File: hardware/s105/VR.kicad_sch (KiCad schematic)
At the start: 18 parts, among them Q19 ., U3 case only

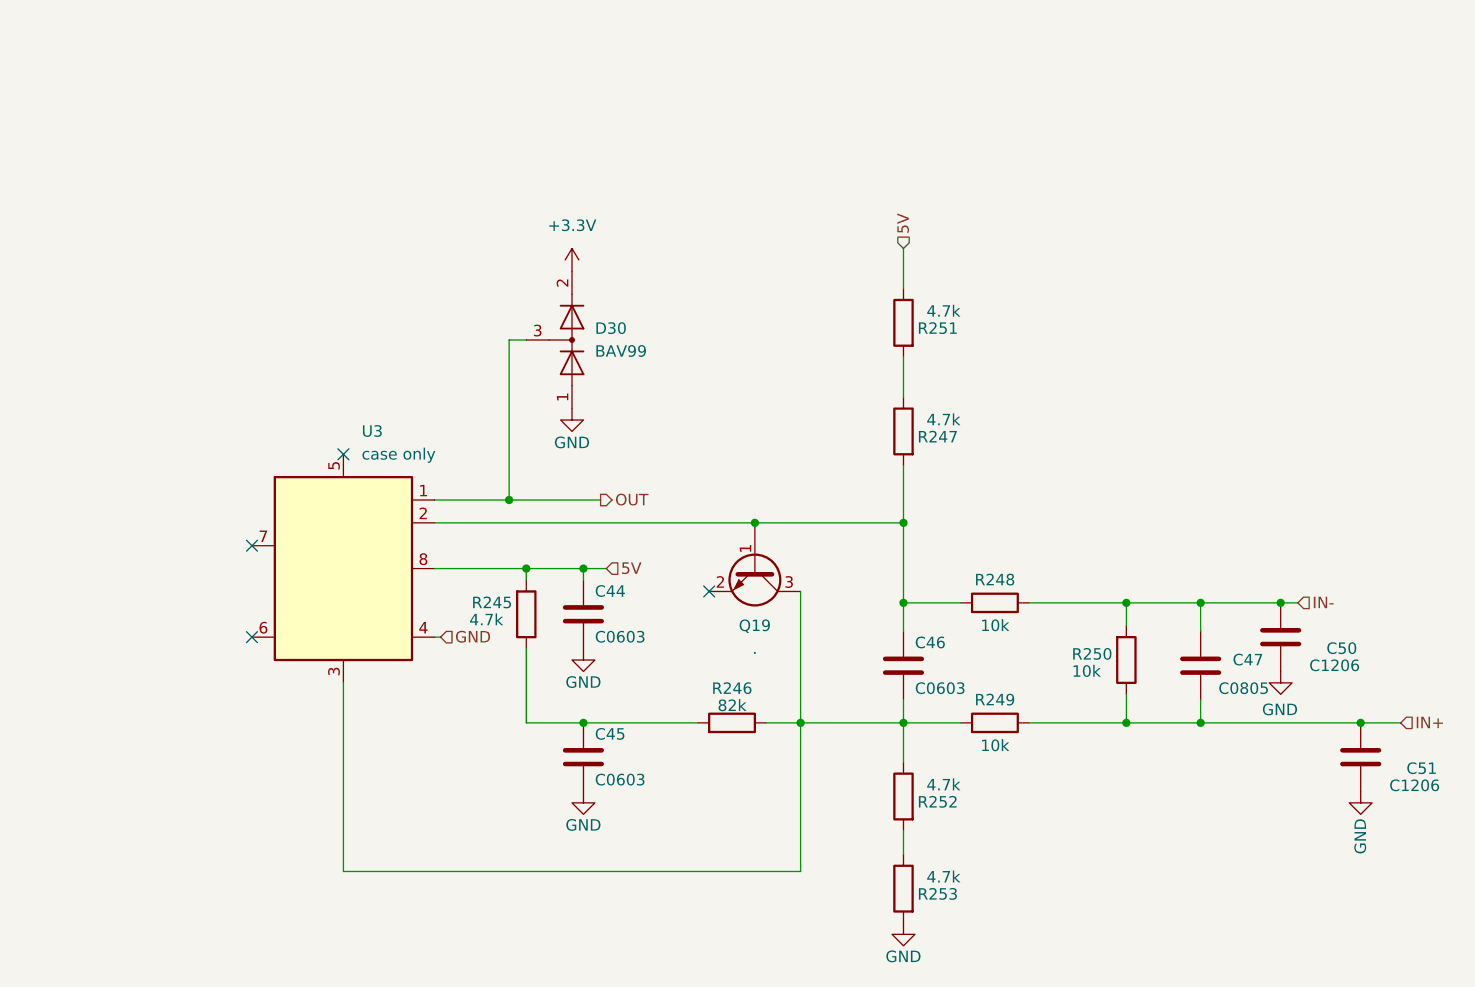
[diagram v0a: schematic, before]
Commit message: #4 #5 #6 #8
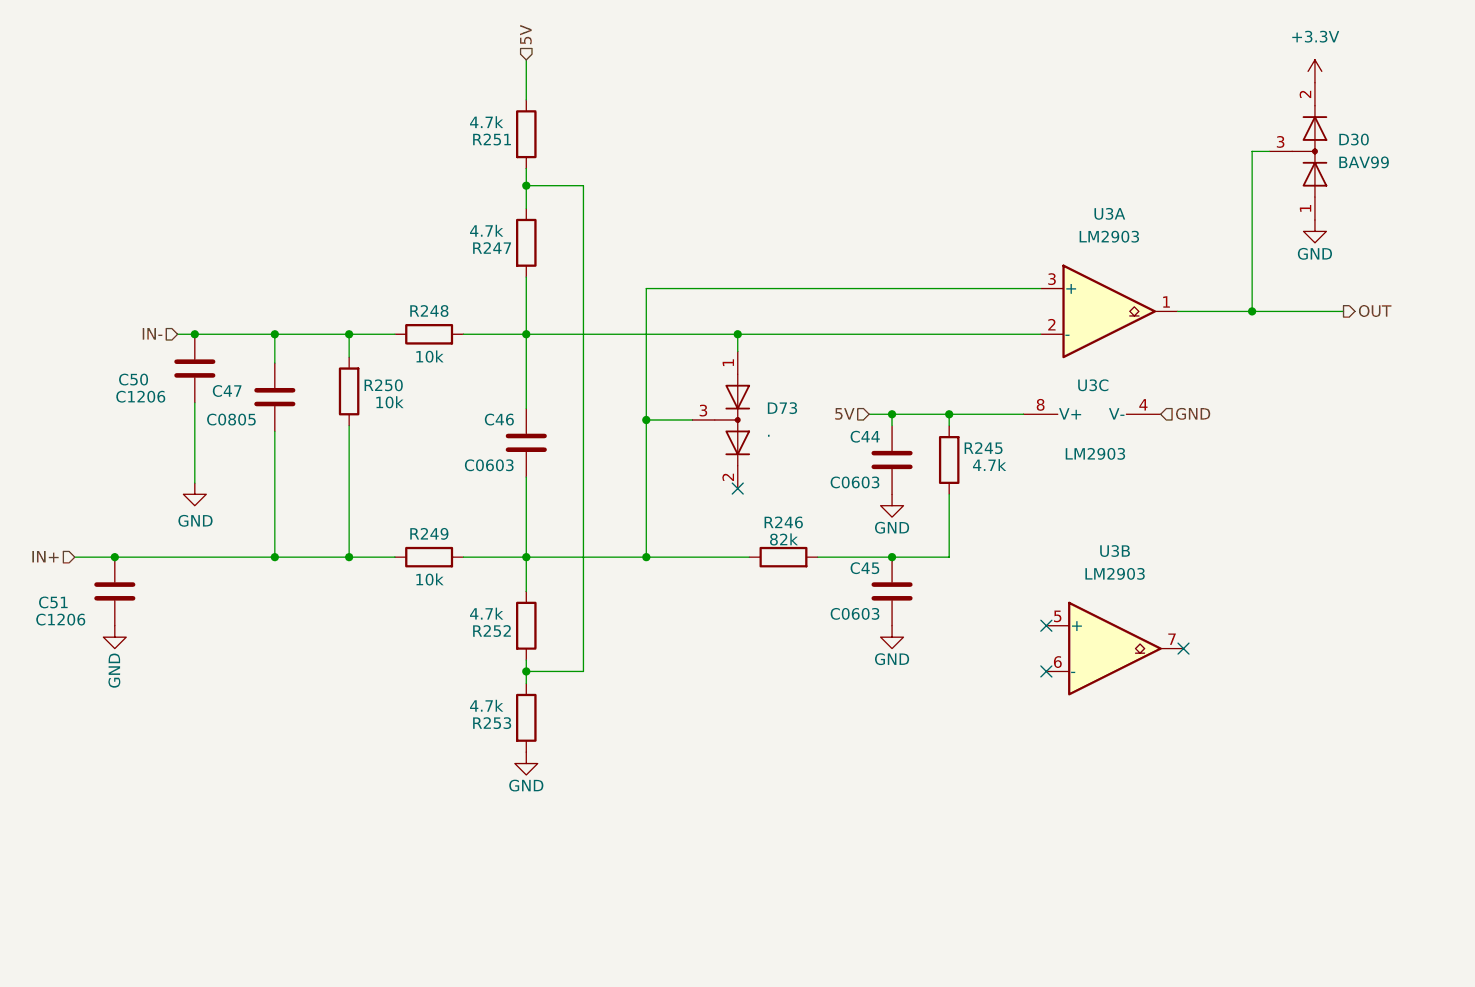
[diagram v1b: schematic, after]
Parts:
- removed Q19: ., Package_TO_SOT_SMD:SOT-23, symbol Transistor_BJT:BC847
- removed U3: case only, Package_SO:SOIC-8_3.9x4.9mm_P1.27mm, symbol Regulator_Controller:L6727
- added D73: ., Package_TO_SOT_SMD:SOT-23, symbol Diode:BAV99
- added U3: LM2903, Package_SO:SOIC-8_3.9x4.9mm_P1.27mm, symbol Comparator:LM2903
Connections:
- net 5V: now also U3.8 (V+)
- net GND: now also U3.4 (V-)
- net OUT: now also U3.1
- net at C46.1, R247.2, R248.2: now also D73.1 (K), U3.2 (-)
- net at C46.2, R246.1, R249.2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: now also D73.3 (K), U3.3 (+)
- net at R252.2, R253.1: now also R247.1, R251.2
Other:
- company: (none) -> rusEFI
- title: (none) -> s105
- moved on the sheet: C44, C45, C46, C47, C50, C51, D30, R245, R246, R247, R248, R249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
